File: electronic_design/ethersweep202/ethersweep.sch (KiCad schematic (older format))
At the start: 88 parts, among them J1 AVR-ISP-6, J10 HR911105A, J2 Conn_01x02_Male, J3 Conn_01x04_Female, J4 Conn_01x02_Male, J5 Conn_01x02_Male, J6 Conn_01x07_Female, J7 Conn_01x07_Male, J8 AVR-ISP-6, M1 Stepper_Motor_bipolar, SW1 SW_Push, U2 ATmega328-AU, U3 DRV8825PWPR, U4 AMS1117-3.3, U5 AS5600, U6 W5500, Y2 Crystal_25MHz, Y3 Crystal

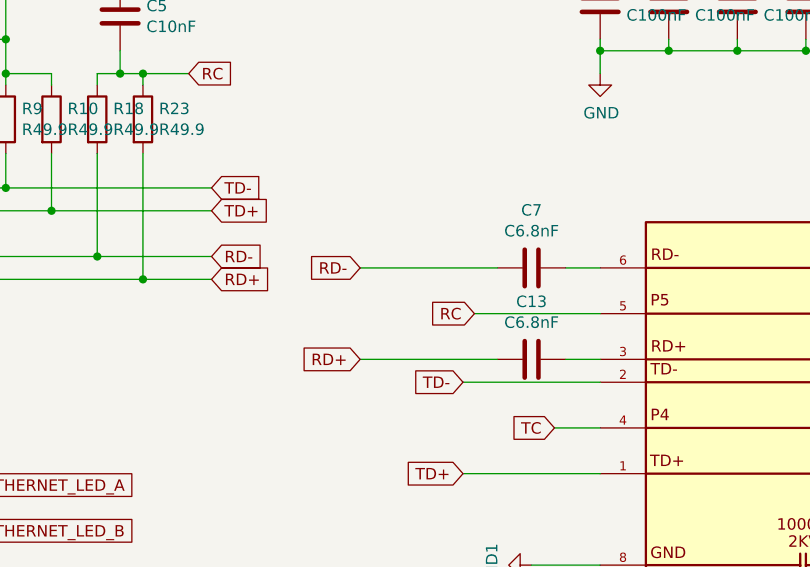
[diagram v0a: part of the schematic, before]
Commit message: design and layout changes
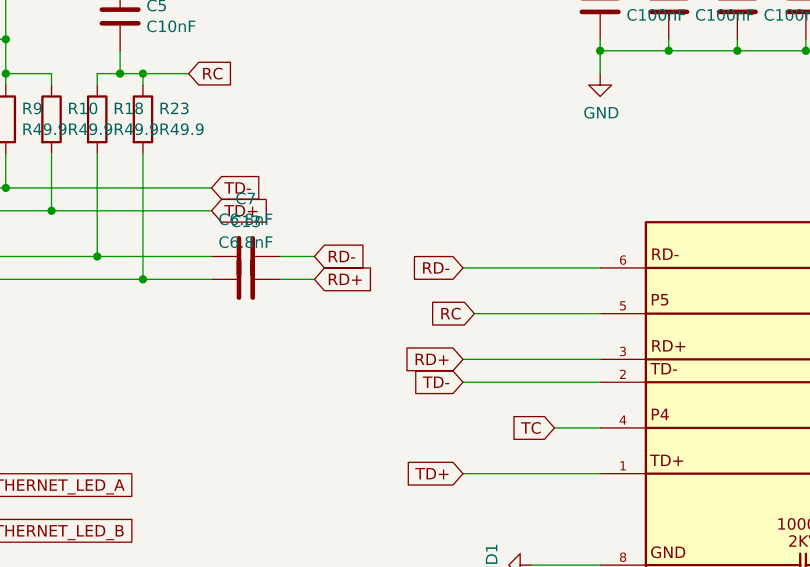
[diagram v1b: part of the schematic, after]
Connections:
- net RD+: now also C13.1, J10.3; no longer C13.2, R23.2, R7.1
- net RD-: now also C7.1, J10.6; no longer C7.2, R18.2, R6.1
- new net: C13.2, R23.2, R7.1
- new net: C7.2, R18.2, R6.1
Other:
- moved on the sheet: C13, C7
